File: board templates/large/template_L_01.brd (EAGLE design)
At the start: 27.9 x 45.7 mm, 2 parts

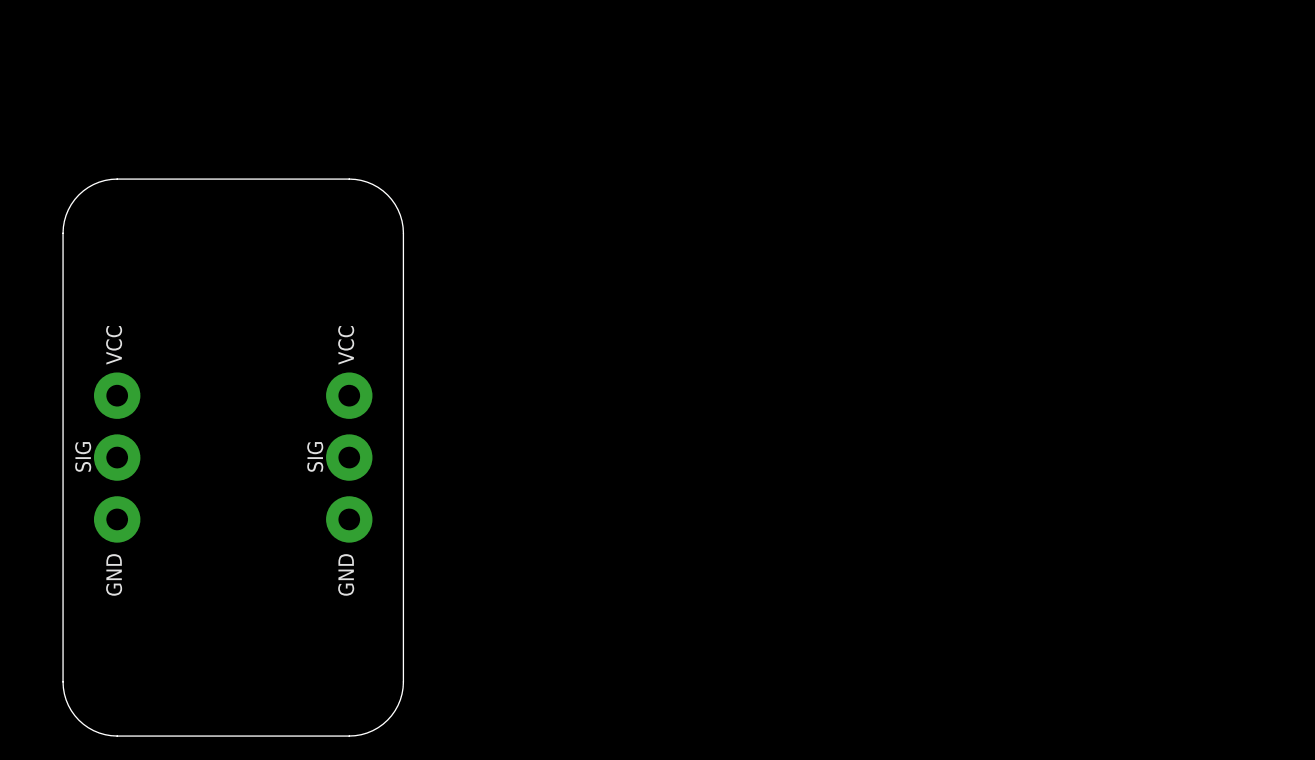
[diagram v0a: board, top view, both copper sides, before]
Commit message: board templates SML
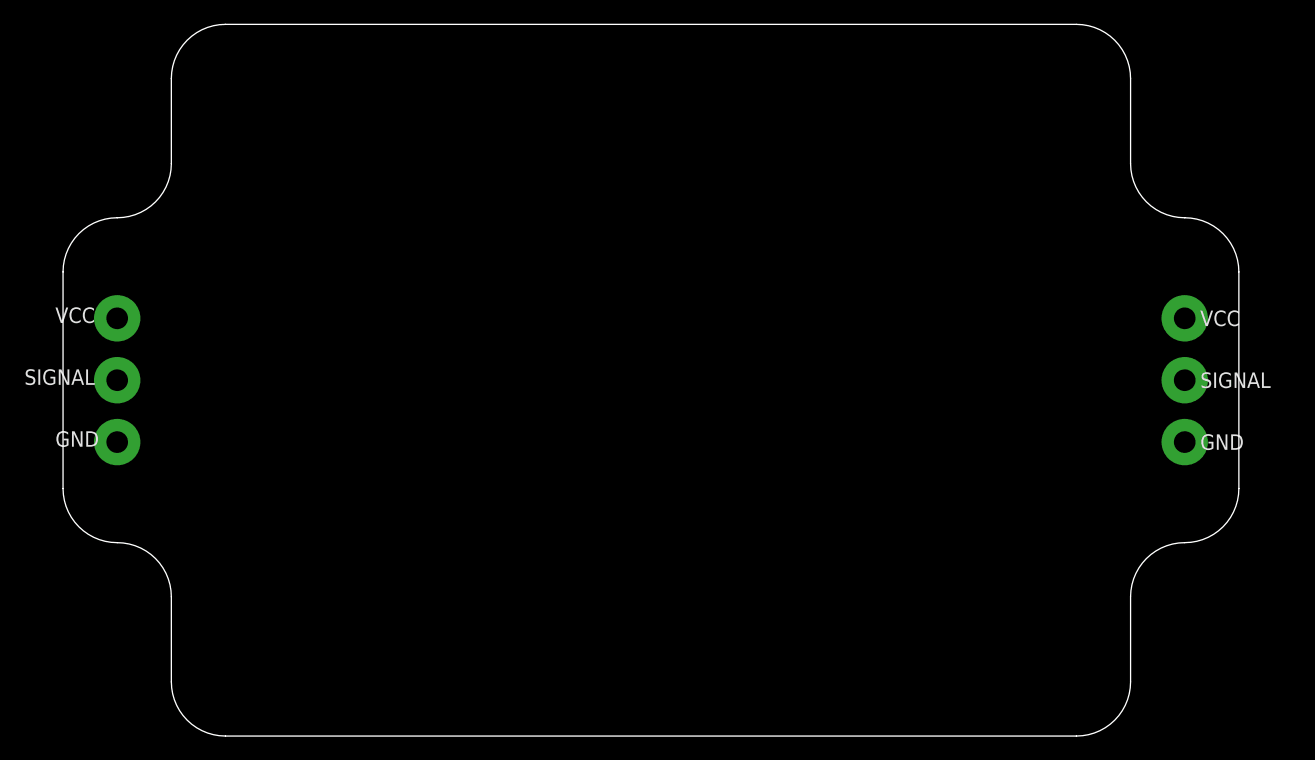
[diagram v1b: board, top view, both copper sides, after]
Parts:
- U$1: value OTHERSNAP-OUTHOLES_ONLY -> OTHERSNAP-OUT; device mentor2:OTHERSNAP-HOLES -> mentor2:OTHERSNAP-OUT
- U$2: value OTHERSNAP-INHOLES_ONLY -> OTHERSNAP-IN; device mentor2:OTHERSNAP-HOLES -> mentor2:OTHERSNAP-IN
- moved U$1 68.9 mm to (92.1, 29.2)
- moved U$2 6.35 mm to (4.45, 29.2)
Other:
- board size 27.9 x 45.7 mm -> 78.7 x 58.4 mm
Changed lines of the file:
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@@
 <setting verticaltext="up"/>
 </settings>
-<grid distance="0.175" unitdist="inch" unit="inch" style="dots" multiple="1" display="yes" altdistance="0.01" altunitdist="mm" altunit="mm"/>
+<grid distance="0.05" unitdist="inch" unit="inch" style="dots" multiple="1" display="yes" altdistance="0.01" altunitdist="mm" altunit="mm"/>
 <layers>
 <layer number="1" name="Top" color="4" fill="1" visible="yes" active="yes"/>
@@
 <board>
 <plain>
-<wire x1="0" y1="41.275" x2="0" y2="4.445" width="0" layer="20"/>
-<wire x1="0" y1="4.445" x2="4.445" y2="0" width="0" layer="20" curve="90"/>
-<wire x1="4.445" y1="0" x2="23.495" y2="0" width="0" layer="20"/>
-<wire x1="23.495" y1="0" x2="27.94" y2="4.445" width="0" layer="20" curve="90"/>
-<wire x1="27.94" y1="4.445" x2="27.94" y2="41.275" width="0" layer="20"/>
-<wire x1="0" y1="41.275" x2="4.445" y2="45.72" width="0" layer="20" curve="-90"/>
-<wire x1="27.94" y1="41.275" x2="23.495" y2="45.72" width="0" layer="20" curve="90"/>
-<wire x1="23.495" y1="45.72" x2="4.445" y2="45.72" width="0" layer="20"/>
+<wire x1="8.89" y1="46.99" x2="8.89" y2="53.975" width="0" layer="20"/>
+<wire x1="8.89" y1="53.975" x2="13.335" y2="58.42" width="0" layer="20" curve="-90"/>
+<wire x1="13.335" y1="58.42" x2="83.185" y2="58.42" width="0" layer="20"/>
+<wire x1="83.185" y1="58.42" x2="87.63" y2="53.975" width="0" layer="20" curve="-90"/>
+<wire x1="87.63" y1="53.975" x2="87.63" y2="46.99" width="0" layer="20"/>
+<wire x1="8.89" y1="11.43" x2="8.89" y2="4.445" width="0" layer="20"/>
+<wire x1="8.89" y1="4.445" x2="13.335" y2="0" width="0" layer="20" curve="90"/>
+<wire x1="87.63" y1="11.43" x2="87.63" y2="4.445" width="0" layer="20"/>
+<wire x1="87.63" y1="4.445" x2="83.185" y2="0" width="0" layer="20" curve="-90"/>
+<wire x1="83.185" y1="0" x2="13.335" y2="0" width="0" layer="20"/>
 </plain>
 <attributes>
@@
 </autorouter>
 <elements>
-<element name="U$1" library="mentor2" package="OTHERSNAP-HOLES" value="OTHERSNAP-OUTHOLES_ONLY" x="23.495" y="22.86"/>
-<element name="U$2" library="mentor2" package="OTHERSNAP-HOLES" value="OTHERSNAP-INHOLES_ONLY" x="4.445" y="22.86"/>
+<element name="U$1" library="mentor2" package="OTHERSNAP-OUT" value="OTHERSNAP-OUT" x="92.075" y="29.21"/>
+<element name="U$2" library="mentor2" package="OTHERSNAP-IN" value="OTHERSNAP-IN" x="4.445" y="29.21"/>
 </elements>
 <signals>
@@
 <contactref element="U$1" pad="GND"/>
 <contactref element="U$2" pad="GND"/>
-<wire x1="4.445" y1="17.78" x2="23.495" y2="17.78" width="0" layer="19" extent="1-1"/>
+<wire x1="4.445" y1="24.13" x2="92.075" y2="24.13" width="0" layer="19" extent="1-1"/>
 </signal>
 <signal name="N$8">
@@
 <contactref element="U$2" pad="VCC"/>
 <contactref element="U$1" pad="VCC"/>
-<wire x1="4.445" y1="27.94" x2="23.495" y2="27.94" width="0" layer="19" extent="1-1"/>
+<wire x1="4.445" y1="34.29" x2="92.075" y2="34.29" width="0" layer="19" extent="1-1"/>
 </signal>
 </signals>
